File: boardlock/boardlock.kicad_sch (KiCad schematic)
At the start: 48 parts, among them U1 ESP32-S3-WROOM-1

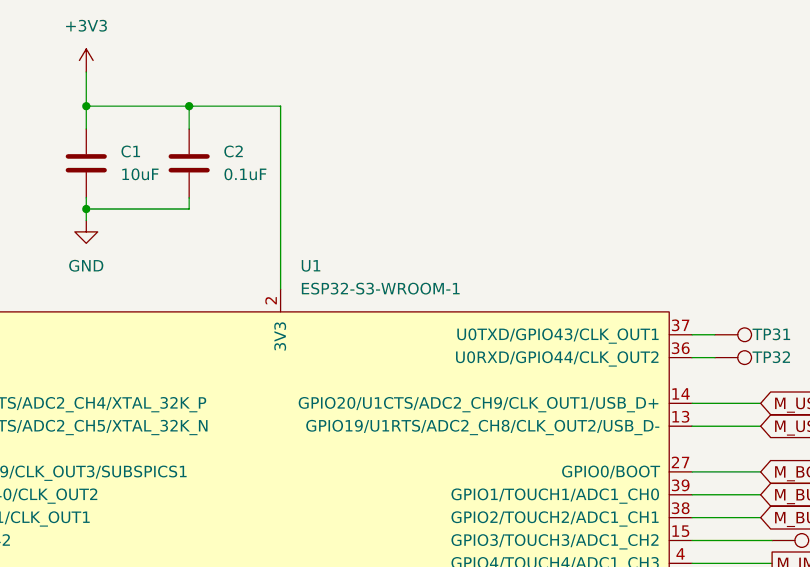
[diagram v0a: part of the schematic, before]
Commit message: footprints finished for now
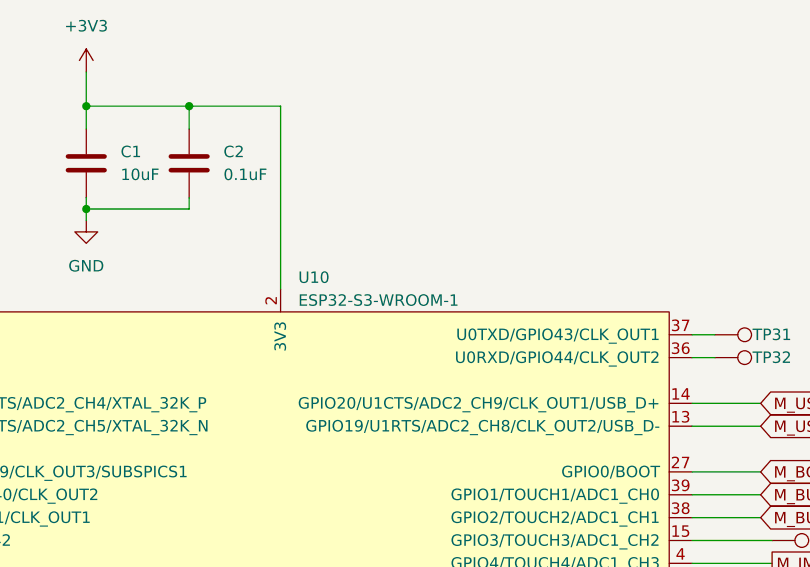
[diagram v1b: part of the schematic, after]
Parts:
- removed U1: ESP32-S3-WROOM-1, PCM_Espressif:ESP32-S3-WROOM-1, symbol PCM_Espressif:ESP32-S3-WROOM-1
- added U10: ESP32-S3-WROOM-1, espressif-kicad:ESP32-S3-WROOM-1, symbol Espressif:ESP32-S3-WROOM-1
- H1, H2, H3, H4: footprint (none) -> MountingHole:MountingHole_2.2mm_M2
- TP10, TP11, TP12, TP13, TP14, TP15, TP16, TP17, TP18, TP19, TP20, TP22, TP23, TP24, TP25, TP26, TP27, TP28, TP29, TP31, TP32, TP35, TP36, TP37, TP38, TP39, TP4, TP41, TP42, TP7, TP8, TP9: footprint (none) -> TestPoint:TestPoint_Pad_D1.0mm
- TP30, TP33, TP34, TP5: footprint TestPoint:TestPoint_Plated_Hole_D3.0mm -> TestPoint:TestPoint_Pad_D1.0mm
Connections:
- net +3V3: now also U10.2 (3V3)
- net GND: now also U10.1 (GND), U10.40 (GND), U10.41 (GND)
- net M_AUDIO_SD_MODE: now also U10.9 (GPIO16/U0CTS/ADC2_CH5/XTAL_32K_N)
- net M_BOOST_EN: now also U10.24 (GPIO47/SPICLK_P/SUBSPICLK_P_DIFF)
- net M_BOOT: now also U10.27 (GPIO0/BOOT)
- net M_BUTTON_EXT1: now also U10.39 (GPIO1/TOUCH1/ADC1_CH0)
- net M_BUTTON_EXT2: now also U10.38 (GPIO2/TOUCH2/ADC1_CH1)
- net M_BUTTON_INT: now also U10.31 (GPIO38/FSPIWP/SUBSPIWP)
- net M_BUZZER: now also U10.25 (GPIO48/SPICLK_N/SUBSPICLK_N_DIFF)
- net M_FUEL_GPOUT: now also U10.8 (GPIO15/U0RTS/ADC2_CH4/XTAL_32K_P)
- net M_GPS_EXTINT: now also U10.23 (GPIO21)
- net M_GPS_POWER: now also U10.22 (GPIO14/TOUCH14/ADC2_CH3/FSPIWP/FSPIDQS/SUBSPIWP)
- net M_HEARTBEAT: now also U10.30 (SPIDQS/GPIO37/FSPIQ/SUBSPIQ)
- net M_I2C_SCL: now also U10.17 (GPIO9/TOUCH9/ADC1_CH8/FSPIHD/SUBSPIHD)
- net M_I2C_SDA: now also U10.12 (GPIO8/TOUCH8/ADC1_CH7/SUBSPICS1)
- net M_I2S_BCLK: now also U10.6 (GPIO6/TOUCH6/ADC1_CH5)
- net M_I2S_Data_Out: now also U10.5 (GPIO5/TOUCH5/ADC1_CH4)
- net M_I2S_LRC: now also U10.7 (GPIO7/TOUCH7/ADC1_CH6)
- net M_IMU_INT2: now also U10.28 (SPIIO6/GPIO35/FSPID/SUBSPID)
- net M_IMU_POWER: now also U10.4 (GPIO4/TOUCH4/ADC1_CH3)
- net M_RGB_B: now also U10.35 (MTMS/GPIO42)
- net M_RGB_G: now also U10.34 (MTDI/GPIO41/CLK_OUT1)
- net M_RGB_R: now also U10.33 (MTDO/GPIO40/CLK_OUT2)
- net M_RST_N: now also U10.3 (EN)
- net M_SPI_CLK: now also U10.20 (GPIO12/TOUCH12/ADC2_CH1/FSPICLK/FSPIIO6/SUBSPICLK)
- net M_SPI_CS: now also U10.18 (GPIO10/TOUCH10/ADC1_CH9/FSPICS0/FSPIIO4/SUBSPICS0)
- net M_SPI_MISO: now also U10.21 (GPIO13/TOUCH13/ADC2_CH2/FSPIQ/FSPIIO7/SUBSPIQ)
- net M_SPI_MOSI: now also U10.19 (GPIO11/TOUCH11/ADC2_CH0/FSPID/FSPIIO5/SUBSPID)
- net M_UART_RX: now also U10.11 (GPIO18/U1RXD/ADC2_CH7/CLK_OUT3)
- net M_UART_TX: now also U10.10 (GPIO17/U1TXD/ADC2_CH6)
- net M_USB_D+: now also U10.14 (GPIO20/U1CTS/ADC2_CH9/CLK_OUT1/USB_D+)
- net M_USB_D-: now also U10.13 (GPIO19/U1RTS/ADC2_CH8/CLK_OUT2/USB_D-)
- net at TP31.1: now also U10.37 (U0TXD/GPIO43/CLK_OUT1)
- net at TP33.1: now also U10.16 (GPIO46)
- net at TP34.1: now also U10.15 (GPIO3/TOUCH3/ADC1_CH2)
- net at TP30.1: now also U10.26 (GPIO45)
- net at TP6.1: now also U10.29 (SPIIO7/GPIO36/FSPICLK/SUBSPICLK)
- net at TP5.1: now also U10.32 (MTCK/GPIO39/CLK_OUT3/SUBSPICS1)
- net at TP32.1: now also U10.36 (U0RXD/GPIO44/CLK_OUT2)

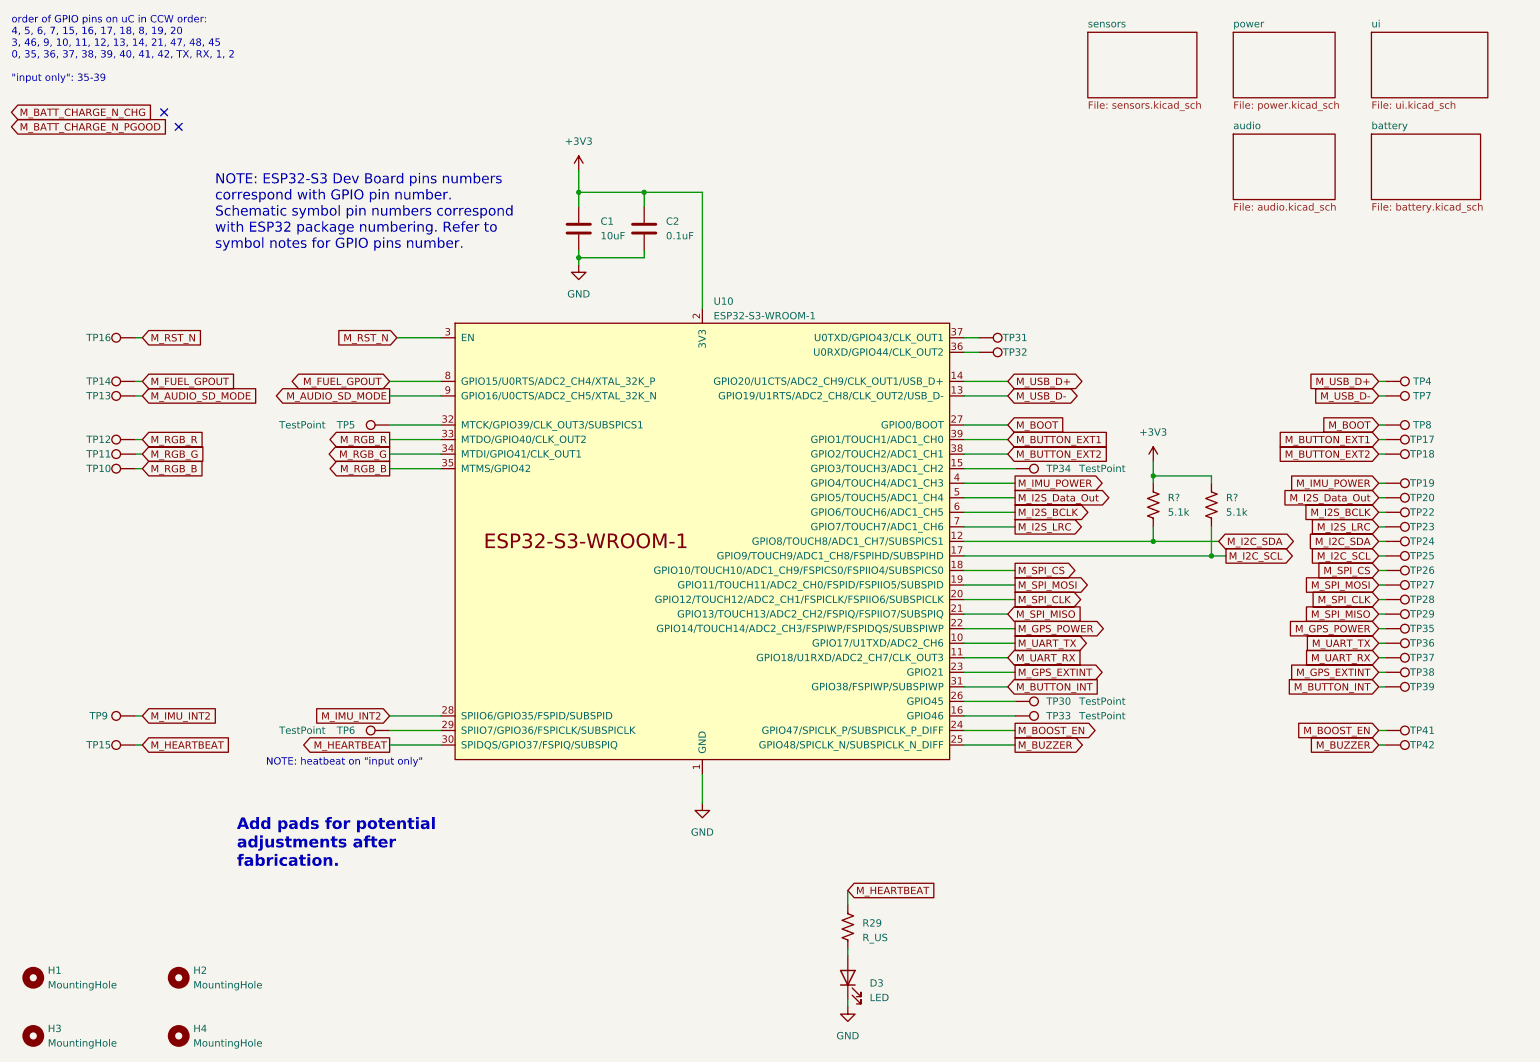
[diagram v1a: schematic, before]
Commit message: Nick PCB edits
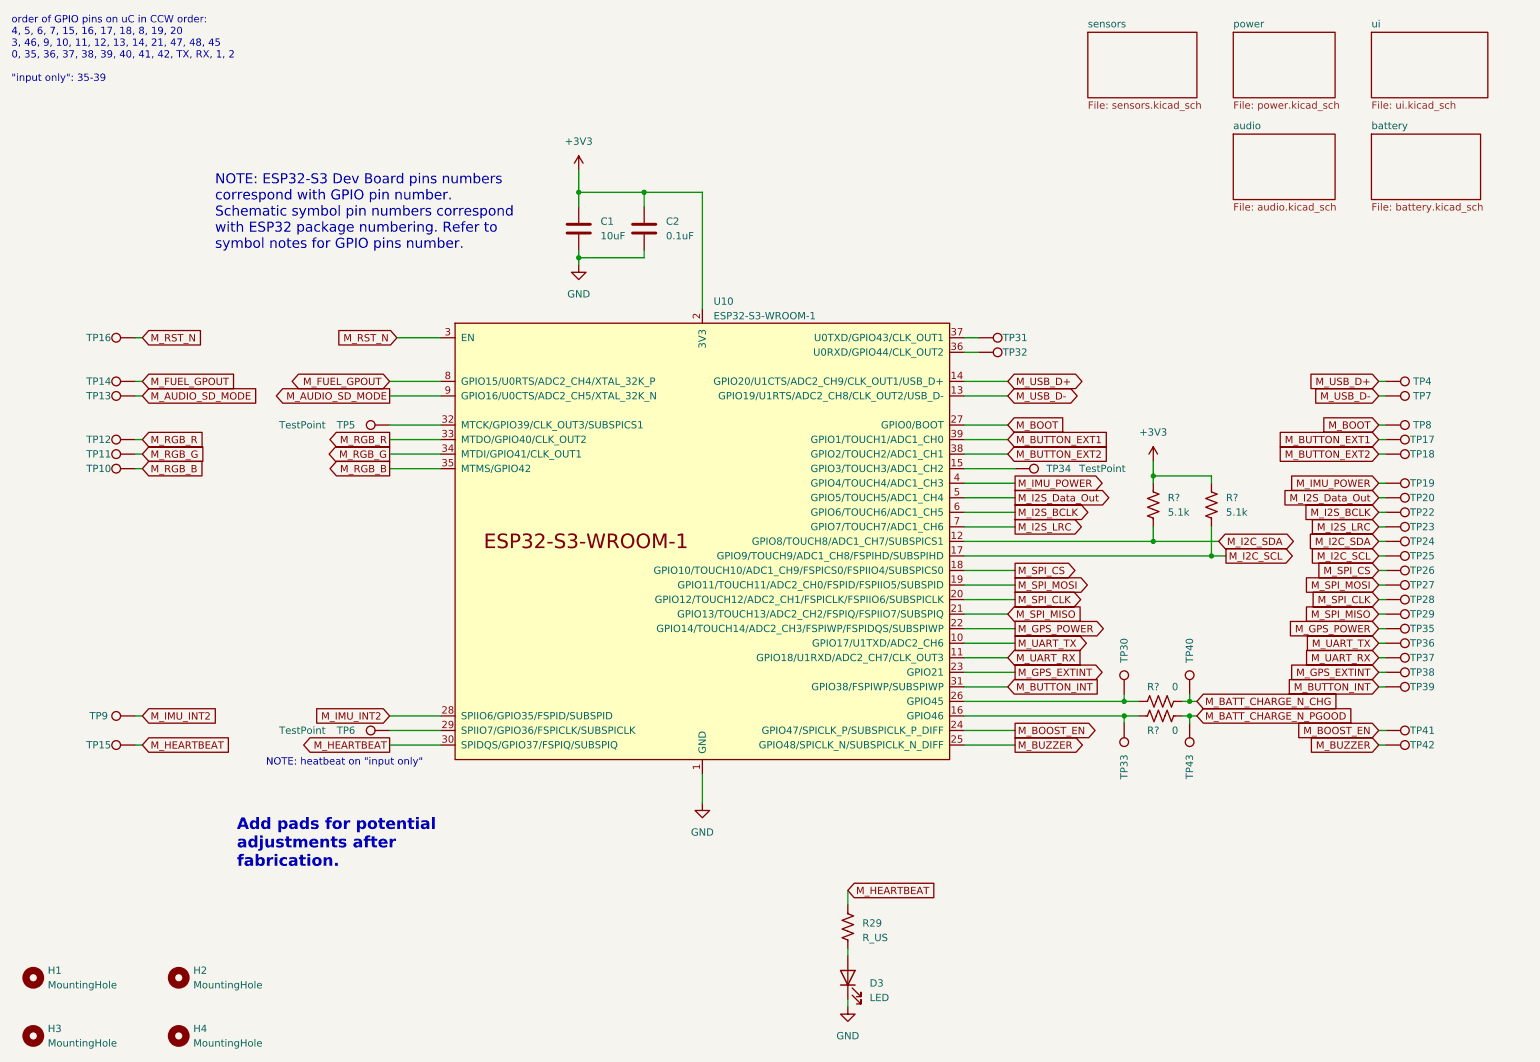
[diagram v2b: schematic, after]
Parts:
- added R? (x2): 0, Resistor_SMD:R_0805_2012Metric_Pad1.20x1.40mm_HandSolder, symbol Device:R_US
- added TP40, TP43: TestPoint, TestPoint:TestPoint_Pad_D1.0mm, symbol Connector:TestPoint
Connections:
- net M_BATT_CHARGE_N_CHG: now also R?.2, TP40.1
- net M_BATT_CHARGE_N_PGOOD: now also R?.2, TP43.1
- net at TP33.1, U10.16 (GPIO46): now also R?.1
- net at TP30.1, U10.26 (GPIO45): now also R?.1
- no-connect marks 2 -> 0
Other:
- moved on the sheet: TP30, TP33
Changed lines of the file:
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@@
   (junction (at 213.36 95.25) (diameter 0) (color 0 0 0 0)
   )
+  (junction (at 208.28 137.16) (diameter 0) (color 0 0 0 0)
+  )
   (junction (at 213.36 106.68) (diameter 0) (color 0 0 0 0)
   )
@@
   (junction (at 124.46 45.72) (diameter 0) (color 0 0 0 0)
   )
+  (junction (at 208.28 134.62) (diameter 0) (color 0 0 0 0)
+  )
+  (junction (at 219.71 134.62) (diameter 0) (color 0 0 0 0)
+  )
   (junction (at 113.03 45.72) (diameter 0) (color 0 0 0 0)
   )
-  (no_connect (at 43.18 34.29))
-  (no_connect (at 40.64 31.75))
+  (junction (at 219.71 137.16) (diameter 0) (color 0 0 0 0)
+  )
   (wire (pts (xy 80.01 142.24) (xy 88.9 142.24))
     (stroke (width 0) (type default))
   )
+  (wire (pts (xy 219.71 134.62) (xy 218.44 134.62))
+    (stroke (width 0) (type default))
+  )
   (wire (pts (xy 180.34 71.12) (xy 182.88 71.12))
     (stroke (width 0) (type default))
   )
+  (wire (pts (xy 220.98 134.62) (xy 219.71 134.62))
+    (stroke (width 0) (type default))
+  )
   (wire (pts (xy 180.34 114.3) (xy 189.23 114.3))
     (stroke (width 0) (type default))
@@
     (stroke (width 0) (type default))
   )
+  (wire (pts (xy 208.28 134.62) (xy 210.82 134.62))
+    (stroke (width 0) (type default))
+  )
   (wire (pts (xy 113.03 45.72) (xy 113.03 48.26))
     (stroke (width 0) (type default))
   )
+  (wire (pts (xy 220.98 137.16) (xy 219.71 137.16))
+    (stroke (width 0) (type default))
+  )
   (wire (pts (xy 180.34 104.14) (xy 189.23 104.14))
     (stroke (width 0) (type default))
@@
     (stroke (width 0) (type default))
   )
+  (wire (pts (xy 219.71 137.16) (xy 219.71 138.43))
+    (stroke (width 0) (type default))
+  )
   (wire (pts (xy 36.83 78.74) (xy 35.56 78.74))
     (stroke (width 0) (type default))
@@
     (stroke (width 0) (type default))
   )
+  (wire (pts (xy 219.71 137.16) (xy 218.44 137.16))
+    (stroke (width 0) (type default))
+  )
+  (wire (pts (xy 208.28 134.62) (xy 208.28 133.35))
+    (stroke (width 0) (type default))
+  )
   (wire (pts (xy 180.34 109.22) (xy 223.52 109.22))
     (stroke (width 0) (type default))
   )
-  (wire (pts (xy 180.34 137.16) (xy 189.23 137.16))
+  (wire (pts (xy 180.34 137.16) (xy 208.28 137.16))
     (stroke (width 0) (type default))
   )
@@
     (stroke (width 0) (type default))
   )
+  (wire (pts (xy 208.28 137.16) (xy 210.82 137.16))
+    (stroke (width 0) (type default))
+  )
   (wire (pts (xy 180.34 142.24) (xy 189.23 142.24))
     (stroke (width 0) (type default))
@@
     (stroke (width 0) (type default))
   )
+  (wire (pts (xy 219.71 134.62) (xy 219.71 133.35))
+    (stroke (width 0) (type default))
+  )
   (wire (pts (xy 252.73 127) (xy 254 127))
     (stroke (width 0) (type default))
@@
     (stroke (width 0) (type default))
   )
-  (wire (pts (xy 180.34 134.62) (xy 189.23 134.62))
+  (wire (pts (xy 180.34 134.62) (xy 208.28 134.62))
+    (stroke (width 0) (type default))
+  )
+  (wire (pts (xy 208.28 137.16) (xy 208.28 138.43))
     (stroke (width 0) (type default))
   )
@@
     )
   )
-  (global_label "M_BATT_CHARGE_N_CHG" (shape input) (at 13.97 31.75 0) (fields_autoplaced)
-    (effects (font (size 1.27 1.27)) (justify left))
-    (property "Intersheetrefs" "${INTERSHEET_REFS}" (at 39.1499 31.75 0)
+  (global_label "M_BATT_CHARGE_N_CHG" (shape input) (at 220.98 134.62 0) (fields_autoplaced)
+    (effects (font (size 1.27 1.27)) (justify left))
+    (property "Intersheetrefs" "${INTERSHEET_REFS}" (at 246.1599 134.62 0)
       (effects (font (size 1.27 1.27)) (justify left) hide)
     )
@@
     )
   )
-  (global_label "M_BATT_CHARGE_N_PGOOD" (shape input) (at 13.97 34.29 0) (fields_autoplaced)
-    (effects (font (size 1.27 1.27)) (justify left))
-    (property "Intersheetrefs" "${INTERSHEET_REFS}" (at 41.7504 34.29 0)
+  (global_label "M_BATT_CHARGE_N_PGOOD" (shape input) (at 220.98 137.16 0) (fields_autoplaced)
+    (effects (font (size 1.27 1.27)) (justify left))
+    (property "Intersheetrefs" "${INTERSHEET_REFS}" (at 248.7604 137.16 0)
       (effects (font (size 1.27 1.27)) (justify left) hide)
     )
@@
     )
   )
-  (symbol (lib_id "Connector:TestPoint") (at 189.23 137.16 270) (unit 1)
-    (in_bom yes) (on_board yes) (dnp no)
-    (property "Reference" "TP33" (at 196.85 137.16 90)
-      (effects (font (size 1.27 1.27)))
-    )
-    (property "Value" "TestPoint" (at 204.47 137.16 90)
-      (effects (font (size 1.27 1.27)))
-    )
-    (property "Footprint" "TestPoint:TestPoint_Pad_D1.0mm" (at 189.23 142.24 0)
-      (effects (font (size 1.27 1.27)) hide)
-    )
-    (property "Datasheet" "~" (at 189.23 142.24 0)
+  (symbol (lib_id "Connector:TestPoint") (at 208.28 138.43 180) (unit 1)
+    (in_bom yes) (on_board yes) (dnp no)
+    (property "Reference" "TP33" (at 208.28 146.05 90)
+      (effects (font (size 1.27 1.27)))
+    )
+    (property "Value" "TestPoint" (at 208.28 153.67 90)
+      (effects (font (size 1.27 1.27)) hide)
+    )
+    (property "Footprint" "TestPoint:TestPoint_Pad_D1.0mm" (at 203.2 138.43 0)
+      (effects (font (size 1.27 1.27)) hide)
+    )
+    (property "Datasheet" "~" (at 203.2 138.43 0)
       (effects (font (size 1.27 1.27)) hide)
     )
@@
     )
   )
+  (symbol (lib_id "Connector:TestPoint") (at 219.71 138.43 180) (unit 1)
+    (in_bom yes) (on_board yes) (dnp no)
+    (property "Reference" "TP43" (at 219.71 146.05 90)
+      (effects (font (size 1.27 1.27)))
+    )
+    (property "Value" "TestPoint" (at 219.71 153.67 90)
+      (effects (font (size 1.27 1.27)) hide)
+    )
+    (property "Footprint" "TestPoint:TestPoint_Pad_D1.0mm" (at 214.63 138.43 0)
+      (effects (font (size 1.27 1.27)) hide)
+    )
+    (property "Datasheet" "~" (at 214.63 138.43 0)
+      (effects (font (size 1.27 1.27)) hide)
+    )
+    (pin "1")
+    (instances
+      (project "boardlock"
+        (path "/e1fc29ce-837e-4062-84d8-c7e423f9eab9"
+          (reference "TP43") (unit 1)
+        )
+      )
+    )
+  )
   (symbol (lib_id "Connector:TestPoint") (at 254 91.44 270) (unit 1)
     (in_bom yes) (on_board yes) (dnp no)
@@
     )
   )
-  (symbol (lib_id "Connector:TestPoint") (at 189.23 134.62 270) (unit 1)
-    (in_bom yes) (on_board yes) (dnp no)
-    (property "Reference" "TP30" (at 196.85 134.62 90)
-      (effects (font (size 1.27 1.27)))
-    )
-    (property "Value" "TestPoint" (at 204.47 134.62 90)
-      (effects (font (size 1.27 1.27)))
-    )
-    (property "Footprint" "TestPoint:TestPoint_Pad_D1.0mm" (at 189.23 139.7 0)
-      (effects (font (size 1.27 1.27)) hide)
-    )
-    (property "Datasheet" "~" (at 189.23 139.7 0)
+  (symbol (lib_id "Connector:TestPoint") (at 208.28 133.35 0) (unit 1)
+    (in_bom yes) (on_board yes) (dnp no)
+    (property "Reference" "TP30" (at 208.28 125.73 90)
+      (effects (font (size 1.27 1.27)))
+    )
+    (property "Value" "TestPoint" (at 208.28 118.11 90)
+      (effects (font (size 1.27 1.27)) hide)
+    )
+    (property "Footprint" "TestPoint:TestPoint_Pad_D1.0mm" (at 213.36 133.35 0)
+      (effects (font (size 1.27 1.27)) hide)
+    )
+    (property "Datasheet" "~" (at 213.36 133.35 0)
       (effects (font (size 1.27 1.27)) hide)
     )
@@
         (path "/e1fc29ce-837e-4062-84d8-c7e423f9eab9"
           (reference "H1") (unit 1)
+        )
+      )
+    )
+  )
+  (symbol (lib_id "Device:R_US") (at 214.63 137.16 90) (unit 1)
+    (in_bom yes) (on_board yes) (dnp no)
+    (property "Reference" "R?" (at 213.36 139.7 90)
+      (effects (font (size 1.27 1.27)))
+    )
+    (property "Value" "0" (at 217.17 139.7 90)
+      (effects (font (size 1.27 1.27)))
+    )
+    (property "Footprint" "Resistor_SMD:R_0805_2012Metric_Pad1.20x1.40mm_HandSolder" (at 214.884 136.144 90)
+      (effects (font (size 1.27 1.27)) hide)
+    )
+    (property "Datasheet" "~" (at 214.63 137.16 0)
+      (effects (font (size 1.27 1.27)) hide)
+    )
+    (pin "1")
+    (pin "2")
+    (instances
+      (project "boardlock"
+        (path "/e1fc29ce-837e-4062-84d8-c7e423f9eab9/a05f4dcd-7a18-4529-a05e-43353e81fbf8"
+          (reference "R?") (unit 1)
+        )
+        (path "/e1fc29ce-837e-4062-84d8-c7e423f9eab9"
+          (reference "R27") (unit 1)
+        )
+      )
+    )
+  )
+  (symbol (lib_id "Connector:TestPoint") (at 219.71 133.35 0) (unit 1)
+    (in_bom yes) (on_board yes) (dnp no)
+    (property "Reference" "TP40" (at 219.71 125.73 90)
+      (effects (font (size 1.27 1.27)))
+    )
+    (property "Value" "TestPoint" (at 219.71 118.11 90)
+      (effects (font (size 1.27 1.27)) hide)
+    )
+    (property "Footprint" "TestPoint:TestPoint_Pad_D1.0mm" (at 224.79 133.35 0)
+      (effects (font (size 1.27 1.27)) hide)
+    )
+    (property "Datasheet" "~" (at 224.79 133.35 0)
+      (effects (font (size 1.27 1.27)) hide)
+    )
+    (pin "1")
+    (instances
+      (project "boardlock"
+        (path "/e1fc29ce-837e-4062-84d8-c7e423f9eab9"
+          (reference "TP40") (unit 1)
         )
       )
@@
         )
       )
+    )
+  )
+  (symbol (lib_id "Device:R_US") (at 214.63 134.62 90) (unit 1)
+    (in_bom yes) (on_board yes) (dnp no)
+    (property "Reference" "R?" (at 213.36 132.08 90)
+      (effects (font (size 1.27 1.27)))
+    )
+    (property "Value" "0" (at 217.17 132.08 90)
+      (effects (font (size 1.27 1.27)))
+    )
+    (property "Footprint" "Resistor_SMD:R_0805_2012Metric_Pad1.20x1.40mm_HandSolder" (at 214.884 133.604 90)
+      (effects (font (size 1.27 1.27)) hide)
+    )
+    (property "Datasheet" "~" (at 214.63 134.62 0)
+      (effects (font (size 1.27 1.27)) hide)
+    )
+    (pin "1")
+    (pin "2")
+    (instances
+      (project "boardlock"
+        (path "/e1fc29ce-837e-4062-84d8-c7e423f9eab9/a05f4dcd-7a18-4529-a05e-43353e81fbf8"
+          (reference "R?") (unit 1)
+        )
+        (path "/e1fc29ce-837e-4062-84d8-c7e423f9eab9"
+          (reference "R26") (unit 1)
+        )
+      )
